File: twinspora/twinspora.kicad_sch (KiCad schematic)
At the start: 149 parts, among them J1 XY-SH1_0-3A61, J2 TYPE-C-31-M-12, J4 Conn_01x02, J5 XY-SH1_0-4A61, J6 Conn_01x02, J7 XY-SH1_0-3A61, J8 XY-SH1_0-3A61, Q1 AO3401A, SW1 SKSGPAE010, SW2 SKSGPAE010, U1 BK22C07-4DP/2-0_4V(800), U10 SRV05-4A, U11 CA-IF1044VD-Q1, U12 ACT1210D-101-2P-TL00, U13 PESD2CAN, U2 BK22C07-4DP/2-0_4V(800), U3 FMMT620TA, U4 WSD4066DN, U5 SMF30CA_C19077519, U6 SRV05-4A, U7 STM32G473RBTx, U8 H5VN10B, U9 XC6206P332MR, X1 X322512MSB4SI

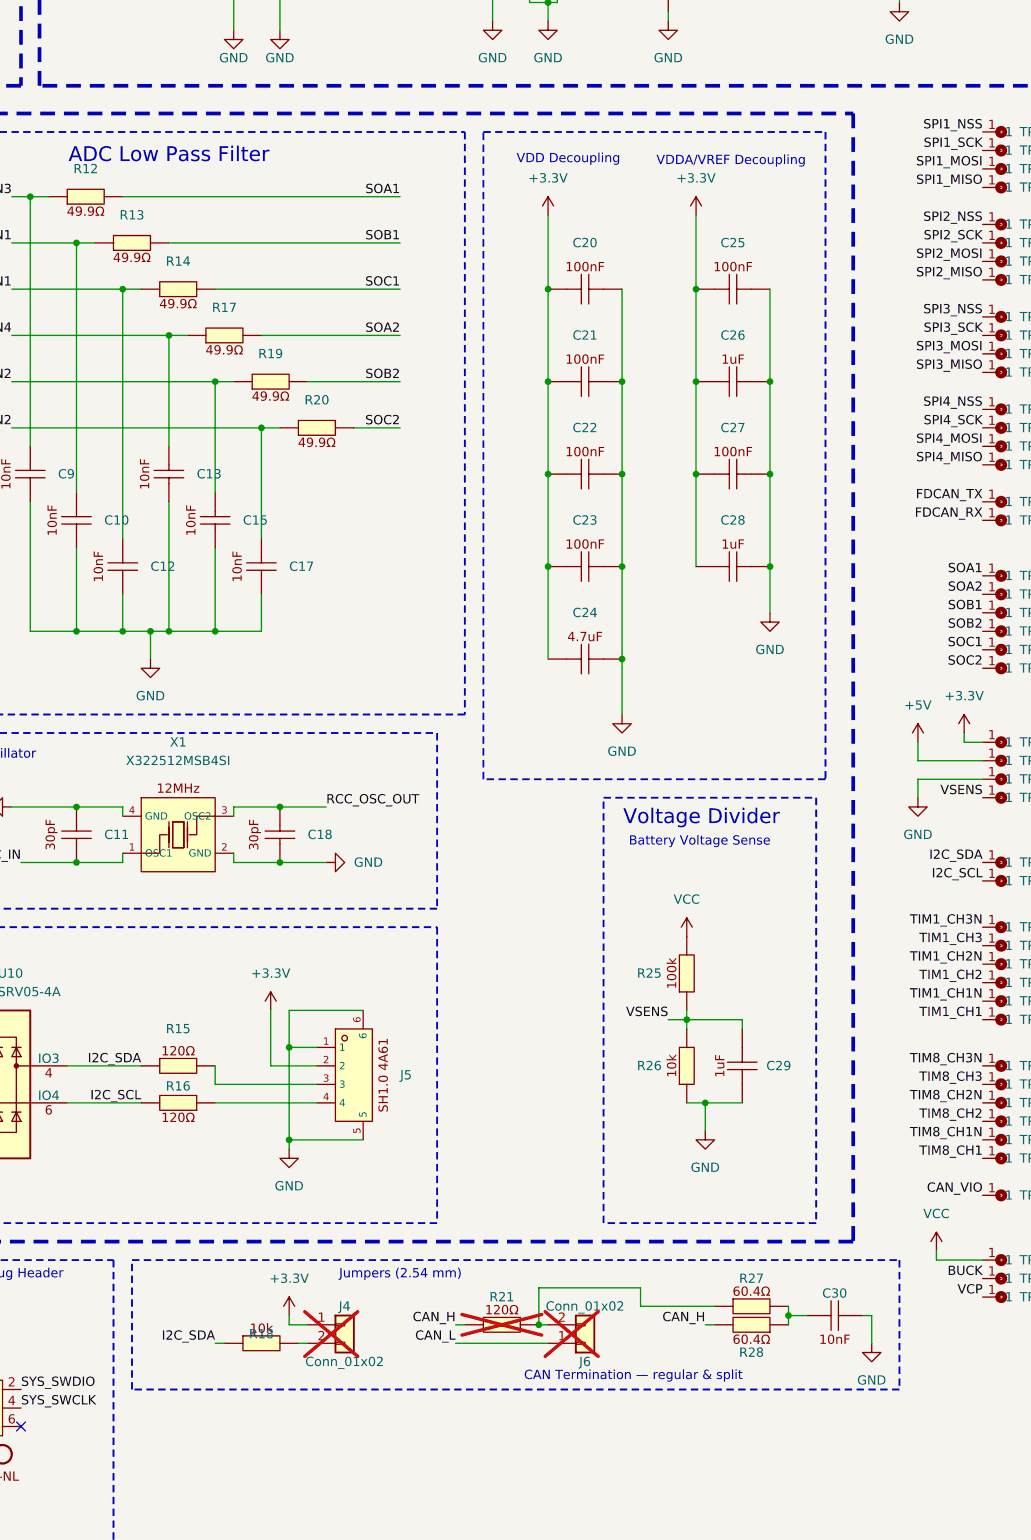
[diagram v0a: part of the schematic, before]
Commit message: fin
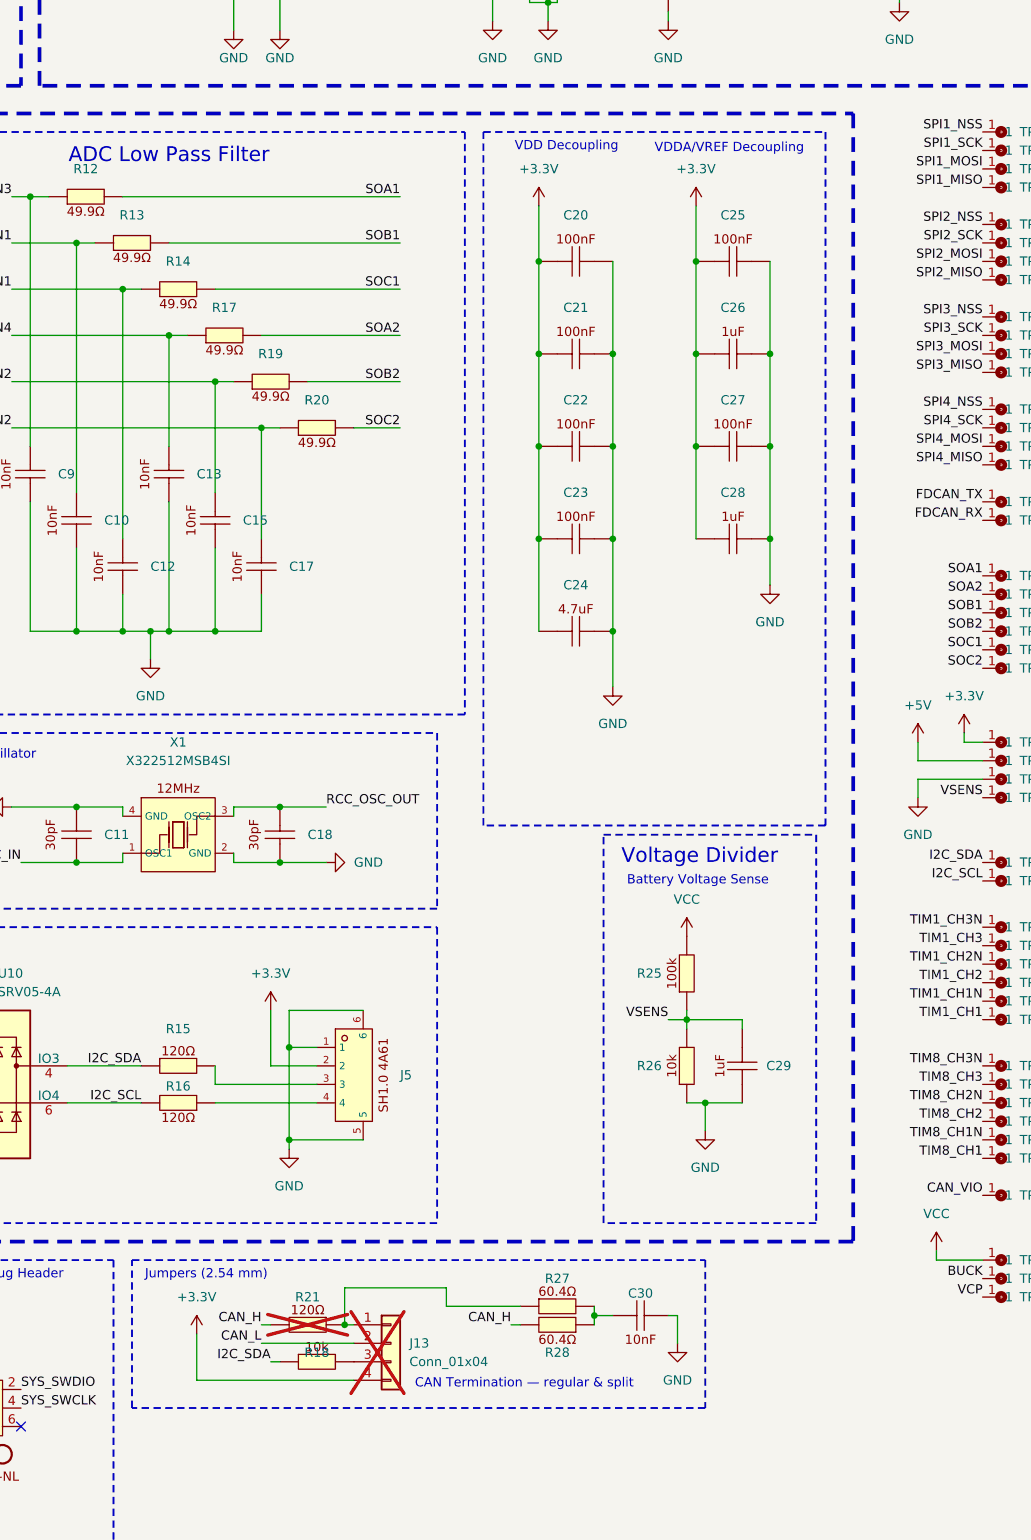
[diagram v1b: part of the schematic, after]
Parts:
- removed J4, J6: Conn_01x02, symbol Connector_Generic:Conn_01x02
- added J13: Conn_01x04, Connector_PinHeader_2.54mm:PinHeader_1x04_P2.54mm_Vertical, symbol Connector_Generic:Conn_01x04
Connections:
- net +3.3V: now also J13.4 (Pin_4)
- net CAN_L: now also J13.2 (Pin_2)
- net at R21.1, R27.1: now also J13.1 (Pin_1)
- net at R18.2: now also J13.3 (Pin_3)
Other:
- moved on the sheet: C20, C21, C22, C23, C24, C25, C26, C27, C28, C30, R18, R21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

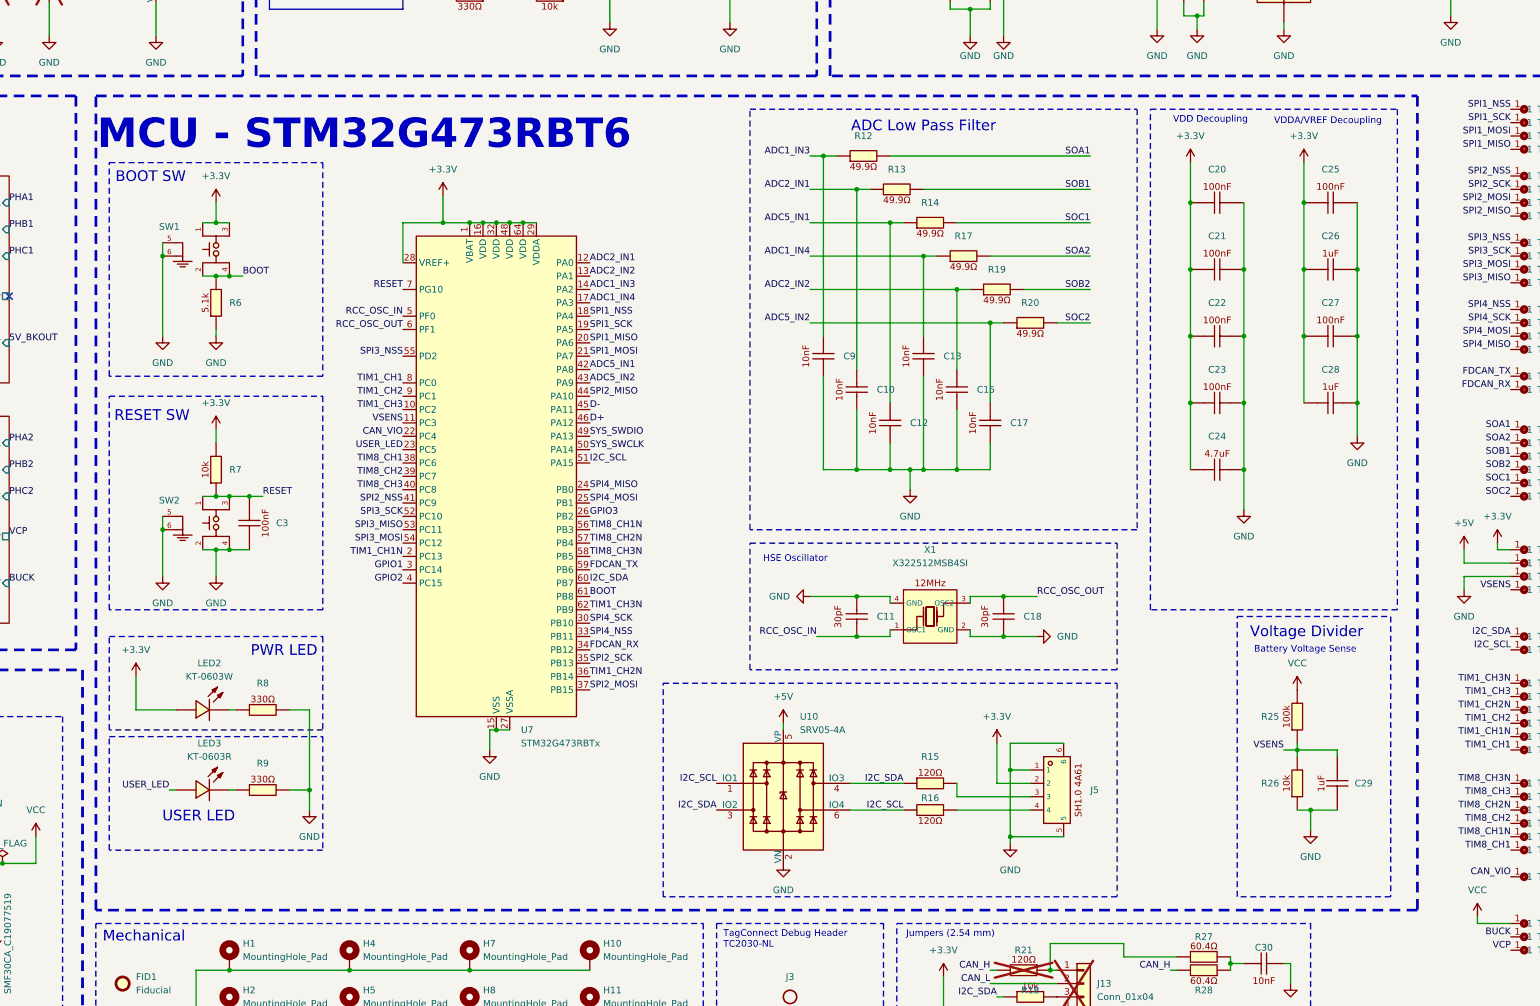
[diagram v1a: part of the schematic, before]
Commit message: ferrite bead
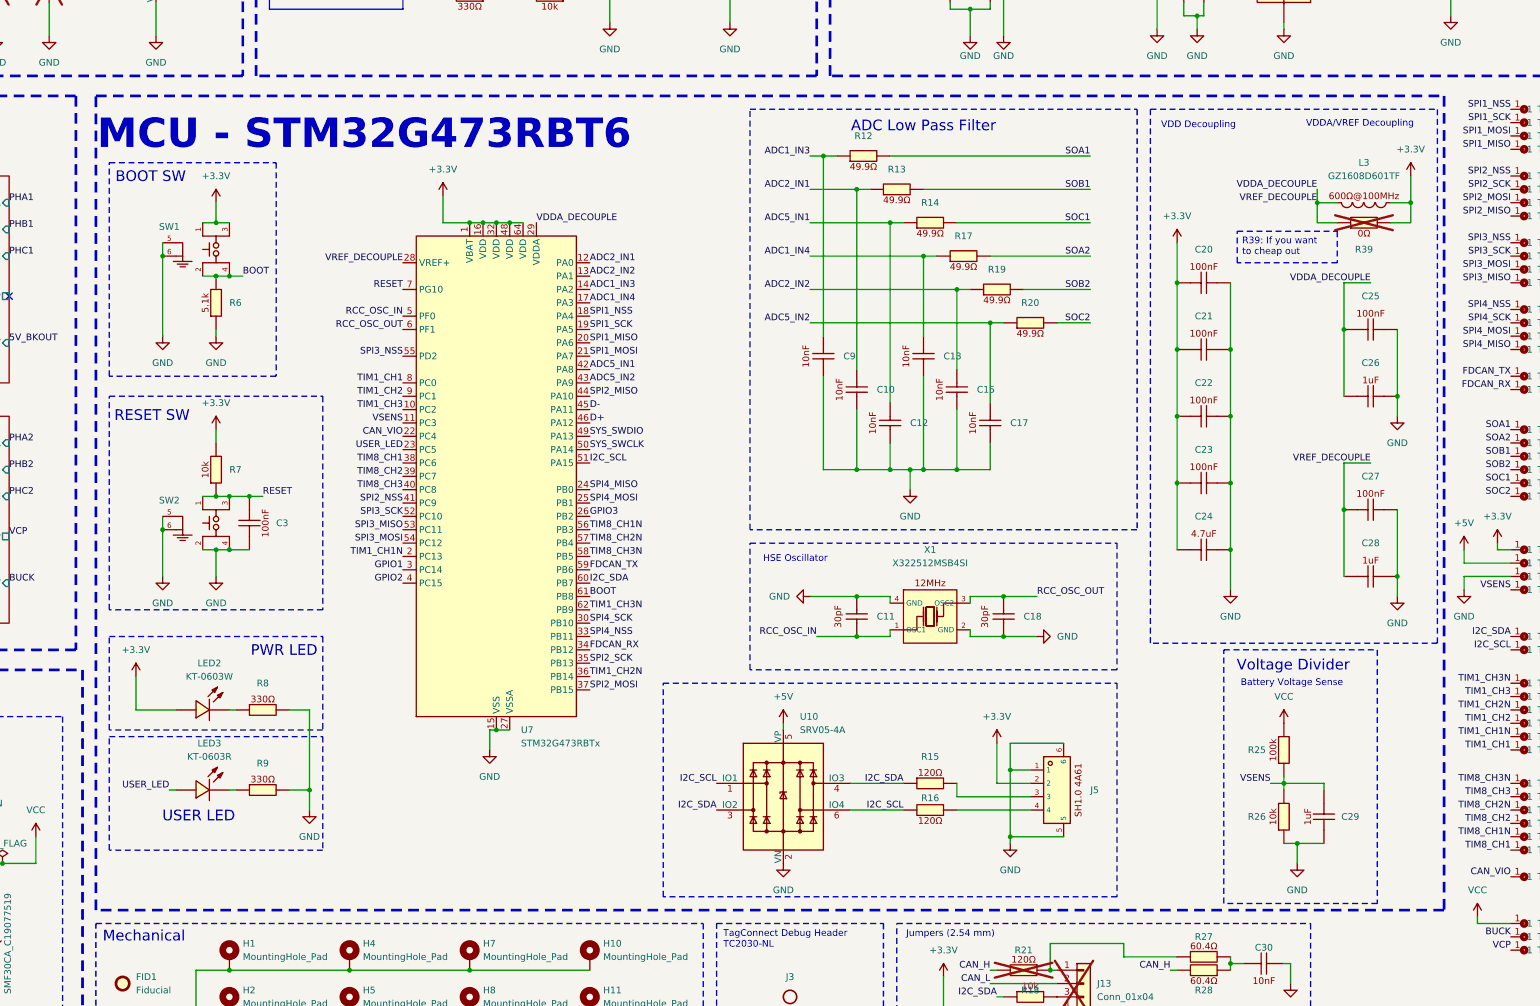
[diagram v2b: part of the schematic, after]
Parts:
- added L3: GZ1608D601TF, Inductor_SMD:L_0603_1608Metric, symbol Inductor__C:GZ1608D601TF
- added R39: 0603WAF0000T5E, Resistor_SMD:R_0603_1608Metric, symbol Basic_Capacitors_Resistors:0603WAF0000T5E
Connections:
- net +3.3V: now also L3.2, R39.2; no longer C25.1, C26.1, C27.1, C28.1, U7.28 (VREF+), U7.29 (VDDA)
- new net VDDA_DECOUPLE: C25.1, C26.1, C27.1, C28.1, L3.1, R39.1, U7.28 (VREF+), U7.29 (VDDA)
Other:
- moved on the sheet: C20, C21, C22, C23, C24, C25, C26, C27, C28, C29, R25, R26
